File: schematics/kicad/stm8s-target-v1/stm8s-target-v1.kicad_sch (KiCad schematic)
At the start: 39 parts, among them J1 ISP_MODE, J10 RESET, J2 VCAP, J3 JMP_3V3, J4 UART, J5 PROGRAM/DEBUG, J6 GPIO, J7 USB_C_Receptacle_USB2.0_16P, J8 Conn_Coaxial, J9 GLITCH_IN, U1 AMS1117-3.3, U2 CH340X, U3 STM8S003F3U

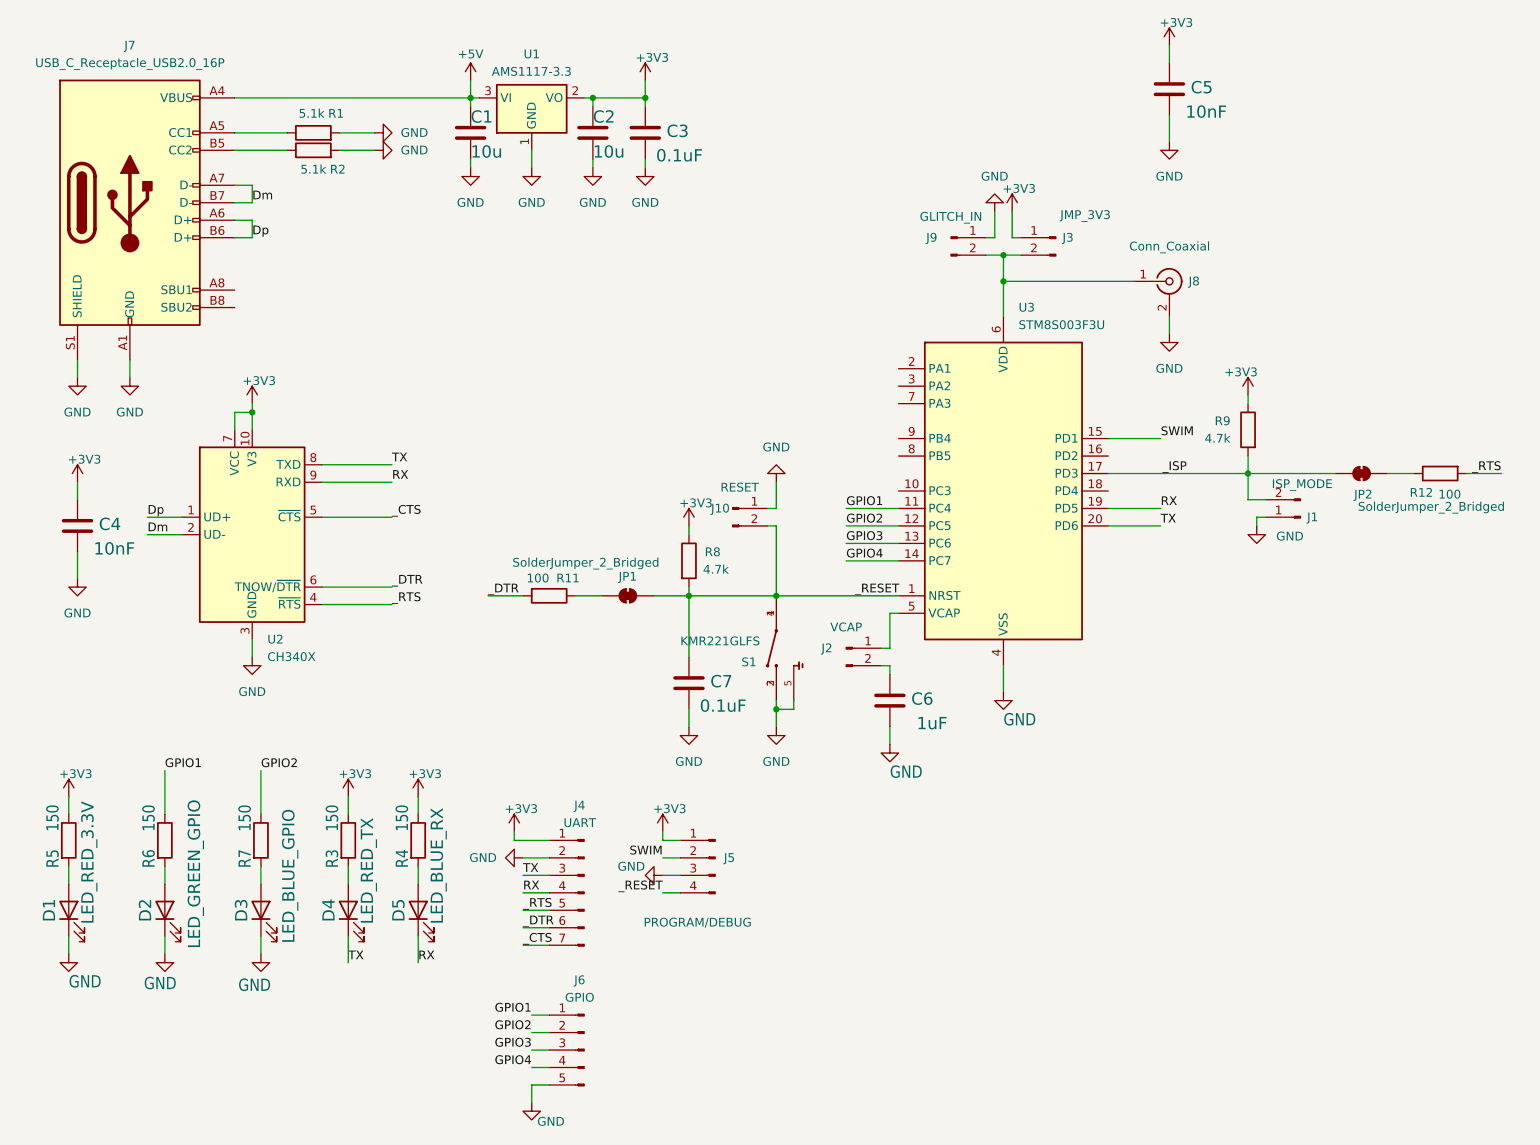
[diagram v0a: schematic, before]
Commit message: refactored findus; renamed scripts (consistent naming scheme); Moved submodules to separate files; fixed an error with arm_multiplexing and the genetic algorithm; added more example scripts; finalized the STM8s target board
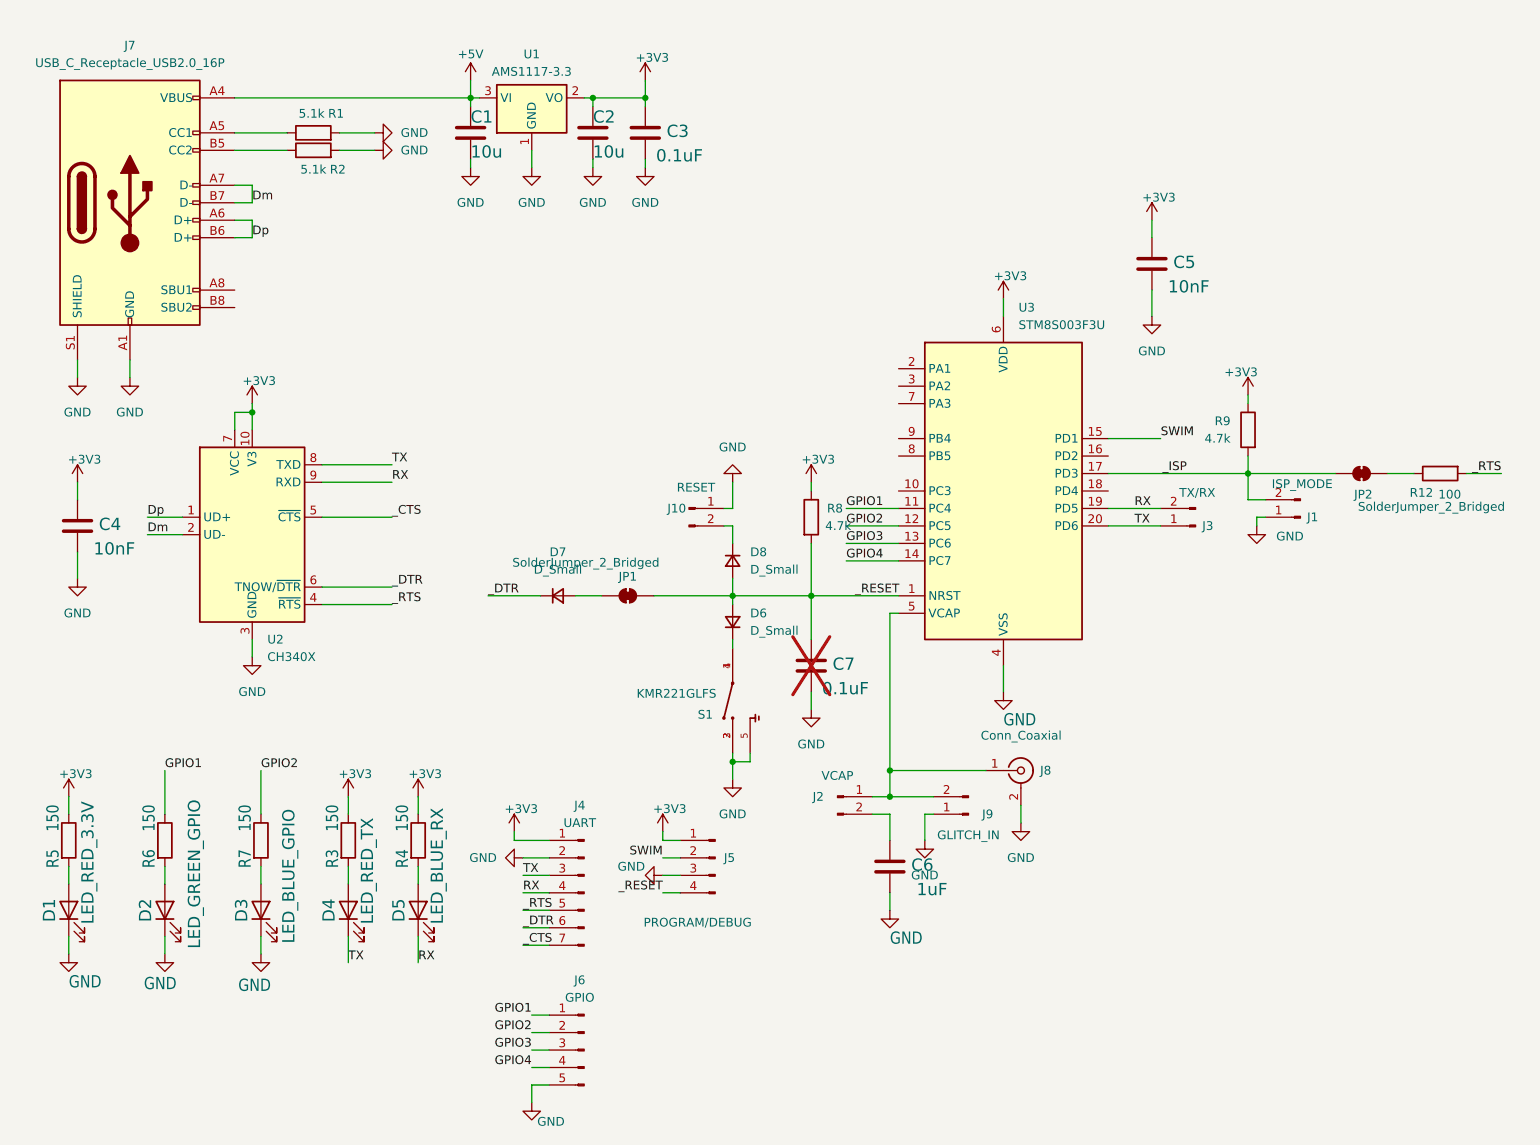
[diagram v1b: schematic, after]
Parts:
- removed R11: 100, Resistor_SMD:R_0603_1608Metric, symbol Device:R
- added D6, D7, D8: D_Small, Diode_SMD:D_SOD-323, symbol Device:D_Small
- C7: now not fitted
- J3: value JMP_3V3 -> TX/RX
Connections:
- net +3V3: now also U3.6 (VDD); no longer J3.1 (Pin_1)
- net RX: now also J3.2 (Pin_2)
- net TX: now also J3.1 (Pin_1)
- net _DTR: now also D7.1 (K)
- net _RESET: now also D6.2 (A), D8.2 (A); no longer J10.2 (Pin_2), S1.1, S1.4
- net at J2.1 (Pin_1), U3.5 (VCAP): now also J8.1 (In), J9.2 (Pin_2)
- net at JP1.1 (A): now also D7.2 (A)
- new net: D8.1 (K), J10.2 (Pin_2)
- new net: D6.1 (K), S1.1, S1.4
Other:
- moved on the sheet: C5, C6, J10, J2, J8, J9, R8, S1
